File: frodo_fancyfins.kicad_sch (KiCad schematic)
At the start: 30 parts, among them J1 Molex MicroFit 2x3, J2 Molex MicroFit 2x3, J3 SWD Header, U1 STM32F072RBTx, U2 MCP2562-E-SN, U3 AZ1117-3.3, Y1 8MHz 12pF

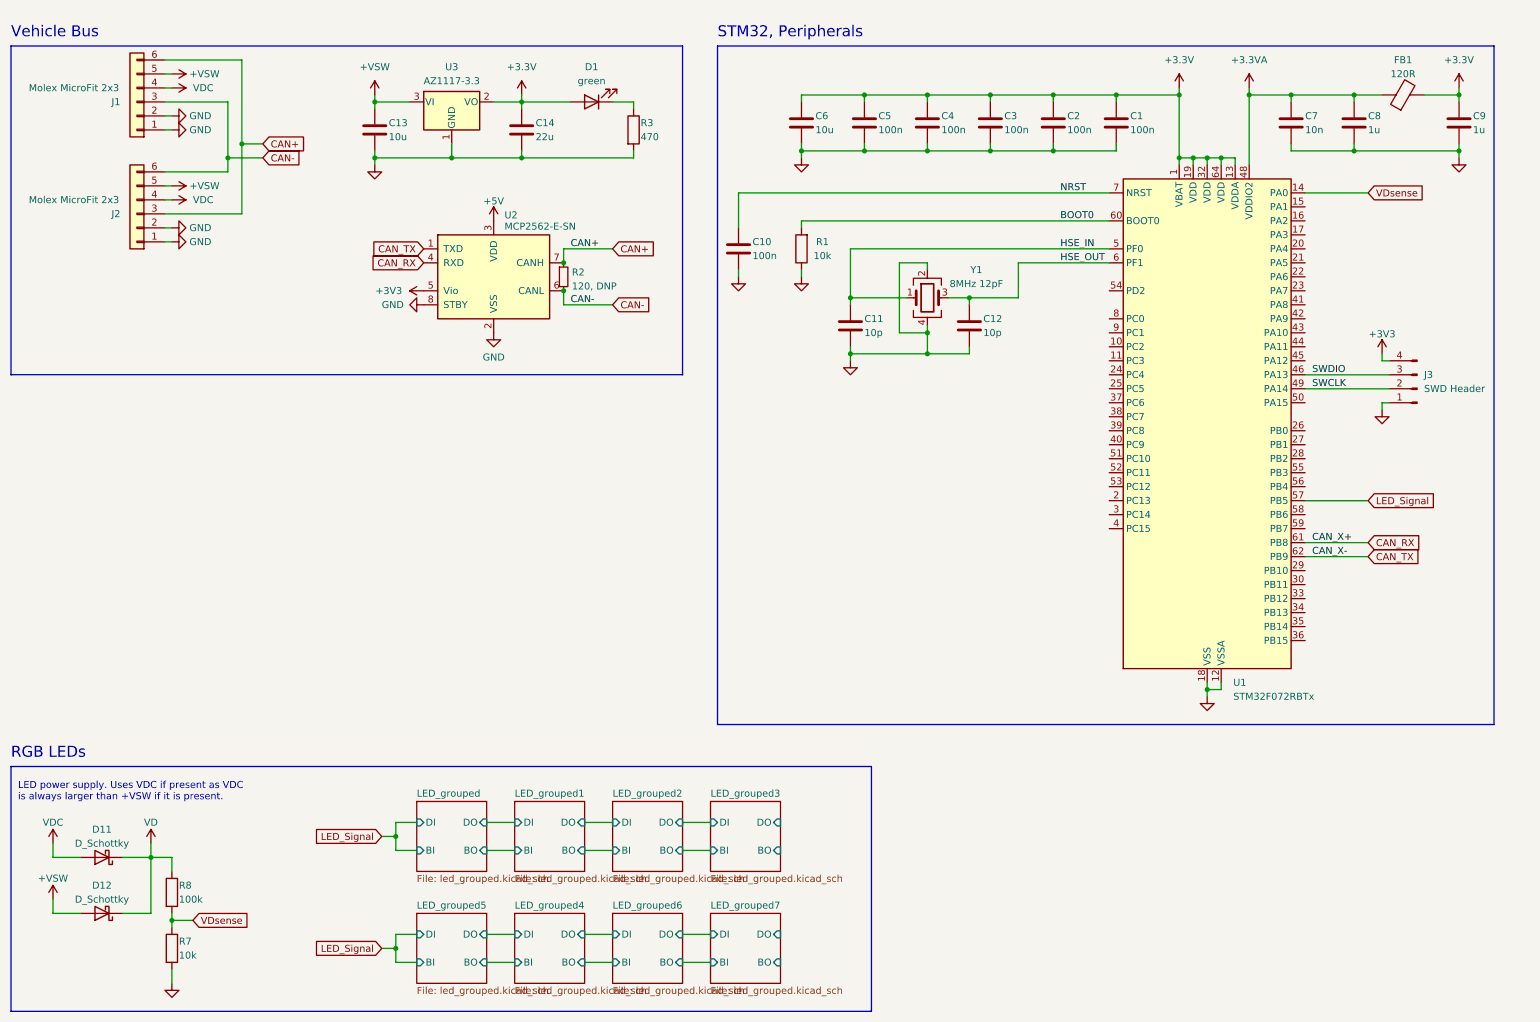
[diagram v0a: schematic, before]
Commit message: Schematics cleanup
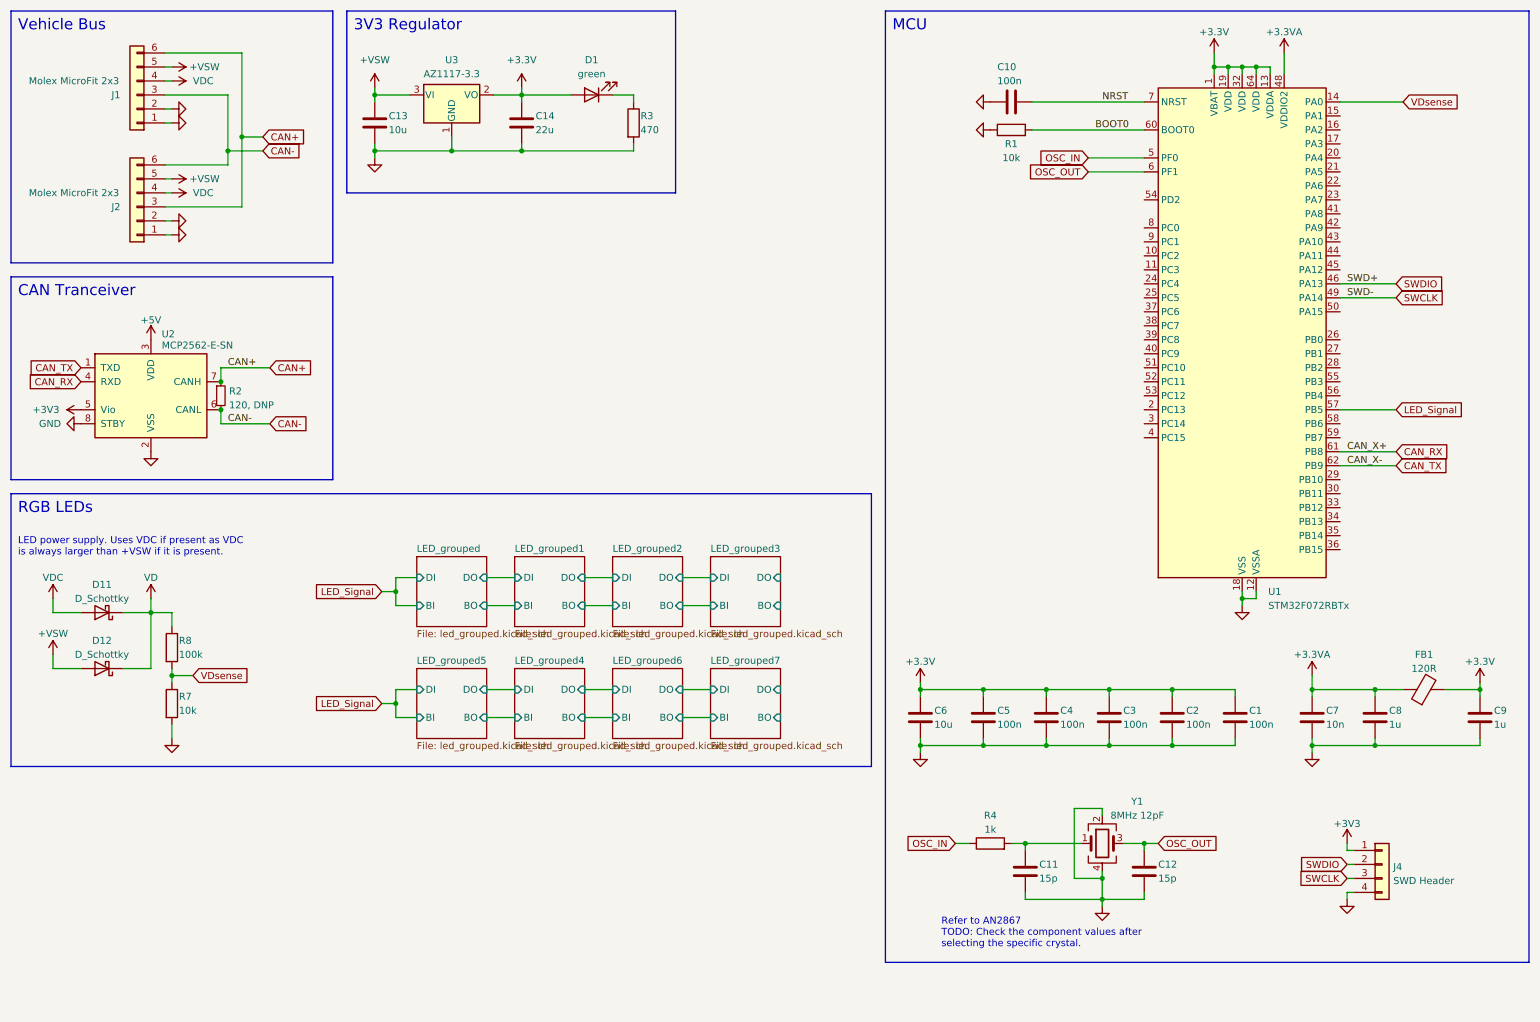
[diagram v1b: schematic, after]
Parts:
- removed J3: SWD Header, symbol Connector:Conn_01x04_Pin
- added J4: SWD Header, Connector_PinHeader_2.54mm:PinHeader_1x04_P2.54mm_Vertical, symbol Connector_Generic:Conn_01x04
- added R4: 1k, symbol Device:R
- C11, C12: value 10p -> 15p
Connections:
- net +3V3: now also J4.1 (Pin_1)
- net GND: now also J4.4 (Pin_4)
- net SWCLK: now also J4.3 (Pin_3)
- net SWDIO: now also J4.2 (Pin_2)
- net HSE_IN: no longer names the net of C11.1, Y1.1
- net HSE_IN: now also R4.2; no longer U1.5 (PF0)
- net HSE_OUT renamed OSC_OUT
- new net OSC_IN: R4.1, U1.5 (PF0)
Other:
- note added: "3V3 Regulator"
- note added: "CAN Tranceiver"
- note added: "MCU"
- note added: "Refer to AN2867 TODO: Check the component values after selecting the specific crystal."
- note removed: "STM32, Peripherals"
- moved on the sheet: C1, C10, C11, C12, C13, C14, C2, C3, C4, C5, C6, C7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
